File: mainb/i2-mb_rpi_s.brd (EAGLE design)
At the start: 110 x 106.6 mm, 27 parts, among them IC3 DS1307Z, T1 BC337, T2 BC337, X9 eth (mb->rpi)

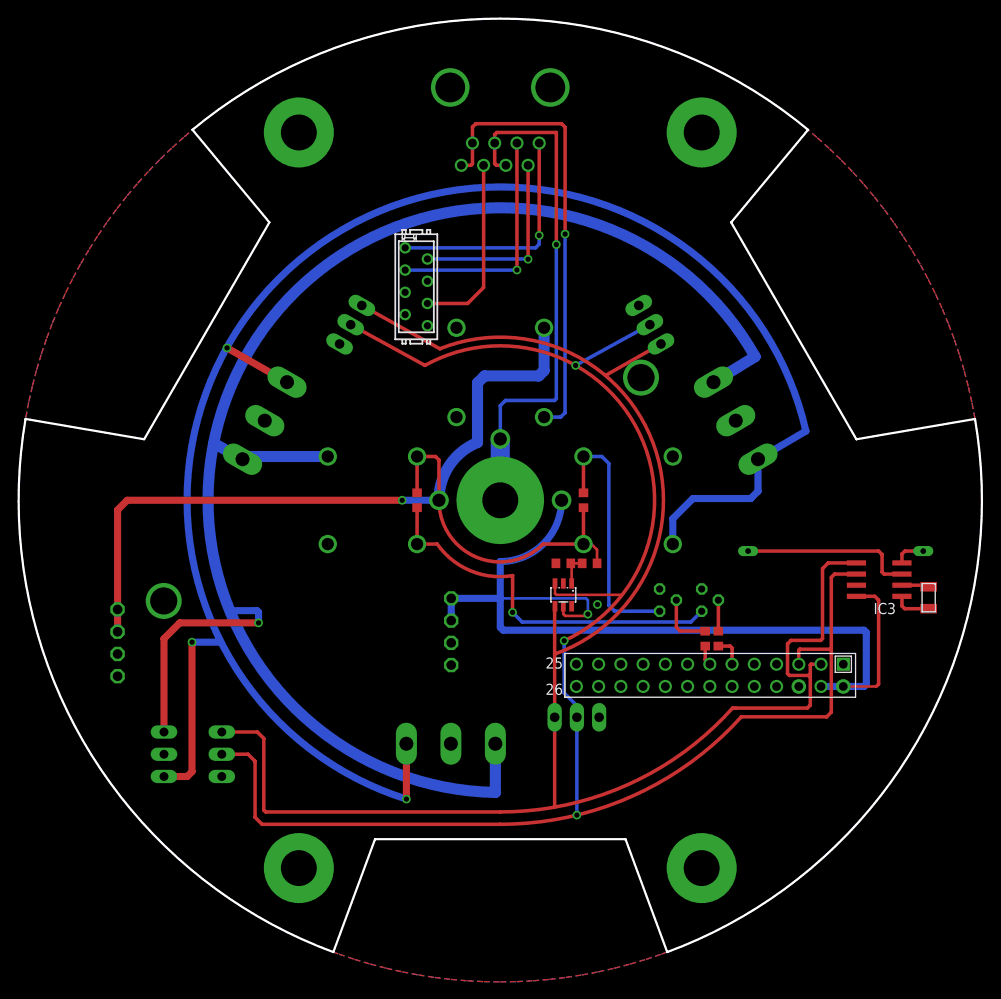
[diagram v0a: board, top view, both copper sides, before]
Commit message: 22.11.13 17:00
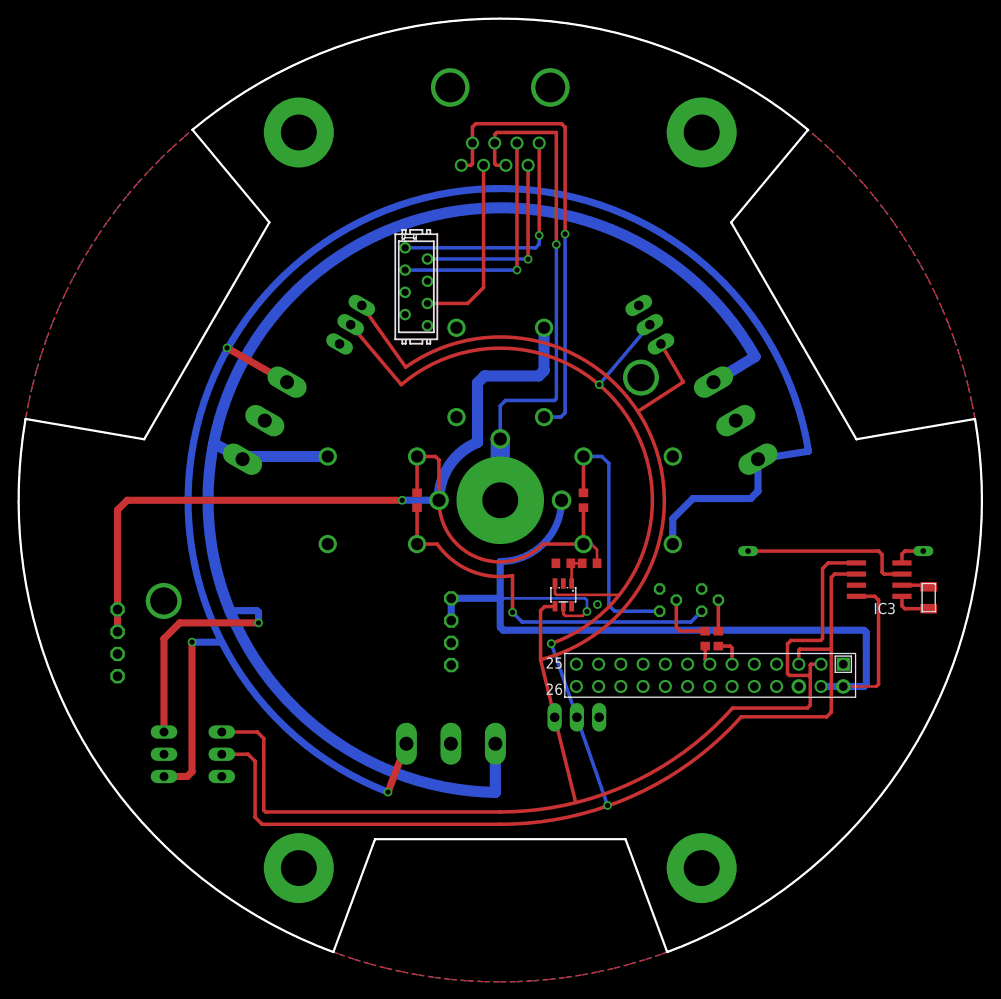
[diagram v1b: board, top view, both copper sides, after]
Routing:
- net SCL: track 200.5 -> 183.5 mm
- net SDA: track 184.4 -> 187.6 mm
- net +5V: track 121.6 -> 120.5 mm
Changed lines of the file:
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@@
 <layer number="46" name="Milling" color="3" fill="1" visible="no" active="yes"/>
 <layer number="47" name="Measures" color="7" fill="1" visible="no" active="yes"/>
-<layer number="48" name="Document" color="7" fill="1" visible="no" active="yes"/>
+<layer number="48" name="Document" color="7" fill="1" visible="yes" active="yes"/>
 <layer number="49" name="Reference" color="7" fill="1" visible="yes" active="yes"/>
 <layer number="50" name="dxf" color="7" fill="1" visible="no" active="no"/>
@@
 <contactref element="I2C_3" pad="2"/>
 <contactref element="I2C_4" pad="2"/>
-<wire x1="-17.0808875" y1="20.049996875" x2="-8.6" y2="15.4" width="0.4064" layer="1"/>
-<wire x1="8.75" y1="-24.78" x2="8.75" y2="-23.45" width="0.4064" layer="16"/>
-<wire x1="7.3" y1="-22" x2="7.3" y2="-16.04" width="0.4064" layer="16"/>
-<wire x1="-8.6" y1="15.4" x2="8.6" y2="15.4" width="0.4064" layer="1" curve="-58.361612"/>
-<wire x1="17.0808875" y1="20.05" x2="8.6" y2="15.4" width="0.4064" layer="16"/>
-<via x="8.6" y="15.4" extent="1-16" drill="0.6"/>
-<wire x1="8.6" y1="15.4" x2="7.3" y2="-16.04" width="0.4064" layer="1" curve="-126.269"/>
-<wire x1="7.3" y1="-22" x2="8.75" y2="-23.45" width="0.4064" layer="16"/>
-<via x="7.3" y="-16.04" extent="1-16" drill="0.6"/>
 <contactref element="I2C_1" pad="2"/>
 <wire x1="-31.8" y1="-29" x2="-28.8" y2="-29" width="0.4064" layer="1"/>
@@
 <wire x1="6.25" y1="-9.4999" x2="6.25" y2="-10.65" width="0.3048" layer="1"/>
 <wire x1="6.25" y1="-10.65" x2="6.4" y2="-10.8" width="0.3048" layer="1"/>
-<wire x1="6.4" y1="-10.8" x2="13.8" y2="-10.8" width="0.3048" layer="1"/>
+<wire x1="6.4" y1="-10.8" x2="13.6" y2="-10.8" width="0.3048" layer="1"/>
 <wire x1="34.09" y1="-18.72" x2="34.09" y2="-17.11" width="0.4064" layer="1"/>
 <wire x1="34.09" y1="-17.11" x2="34.2" y2="-17" width="0.4064" layer="1"/>
 <wire x1="34.2" y1="-17" x2="37.8" y2="-17" width="0.4064" layer="1"/>
 <wire x1="37.8" y1="-17" x2="37.8" y2="-24.2" width="0.4064" layer="1"/>
-<wire x1="8.75" y1="-24.78" x2="8.75" y2="-35.85" width="0.4064" layer="16"/>
+<wire x1="8.75" y1="-24.78" x2="12.25" y2="-34.85" width="0.4064" layer="16"/>
 <wire x1="37.27" y1="-24.73" x2="27.52" y2="-24.73" width="0.4064" layer="1"/>
 <wire x1="0" y1="-37" x2="27.52" y2="-24.73" width="0.4064" layer="1" curve="48.0587"/>
@@
 <wire x1="37.8" y1="-8.8" x2="38.175" y2="-8.425" width="0.4064" layer="1"/>
 <wire x1="40.67" y1="-8.425" x2="38.175" y2="-8.425" width="0.4064" layer="1"/>
-<via x="8.75" y="-35.95" extent="1-16" drill="0.6"/>
-<wire x1="8.75" y1="-35.85" x2="8.75" y2="-35.95" width="0" layer="19" extent="16-16"/>
-<wire x1="6.4" y1="-10.8" x2="7.3" y2="-16.04" width="0" layer="19" extent="1-16"/>
-<wire x1="0" y1="-37" x2="8.75" y2="-35.95" width="0" layer="19" extent="1-1"/>
+<via x="12.25" y="-34.85" extent="1-16" drill="0.6"/>
+<wire x1="-17.0808875" y1="20.049996875" x2="-11.3" y2="13.2" width="0.4064" layer="1"/>
+<wire x1="17.0808875" y1="20.05" x2="11.3" y2="13.2" width="0.4064" layer="16"/>
+<wire x1="8.75" y1="-24.78" x2="5.82" y2="-16.37" width="0.4064" layer="16"/>
+<wire x1="-11.3" y1="13.2" x2="5.82" y2="-16.37" width="0.4064" layer="1" curve="-200.979"/>
+<via x="5.82" y="-16.37" extent="1-16" drill="0.6"/>
+<via x="11.3" y="13.2" extent="1-16" drill="0.6"/>
+<wire x1="-11.3" y1="13.2" x2="11.3" y2="13.2" width="0" layer="19" extent="1-16"/>
+<wire x1="6.4" y1="-10.8" x2="5.82" y2="-16.37" width="0" layer="19" extent="1-16"/>
+<wire x1="0" y1="-37" x2="12.25" y2="-34.85" width="0" layer="19" extent="1-1"/>
 </signal>
 <signal name="SDA">
@@
 <contactref element="I2C_3" pad="1"/>
 <contactref element="I2C_4" pad="1"/>
-<wire x1="6.21" y1="-24.78" x2="6.21" y2="-17.5650875" width="0.4064" layer="1"/>
-<wire x1="6.21" y1="-17.5650875" x2="6.21" y2="-12.1401" width="0.4064" layer="1"/>
-<wire x1="-15.8108875" y1="22.249703125" x2="-6.9" y2="17.3" width="0.4064" layer="1"/>
-<wire x1="18.3508875" y1="17.85029375" x2="12.1" y2="14.3" width="0.4064" layer="1"/>
-<wire x1="-6.9" y1="17.3" x2="6.21" y2="-17.5650875" width="0.4064" layer="1" curve="-182.32"/>
 <contactref element="I2C_1" pad="1"/>
 <wire x1="-31.8" y1="-26.46" x2="-27.74" y2="-26.46" width="0.4064" layer="1"/>
@@
 <wire x1="35.4" y1="-18.8" x2="35.4" y2="-20.2" width="0.4064" layer="1"/>
 <wire x1="35.4" y1="-20.2" x2="35.4" y2="-23.4" width="0.4064" layer="1"/>
-<wire x1="35.07" y1="-23.73" x2="26.92" y2="-23.73" width="0.4064" layer="1"/>
+<wire x1="35.07" y1="-23.73" x2="26.524365625" y2="-23.73" width="0.4064" layer="1"/>
 <wire x1="0" y1="-35.59" x2="26.5231375" y2="-23.731228125" width="0.4064" layer="1" curve="48.17983"/>
 <wire x1="35.07" y1="-23.73" x2="35.4" y2="-23.4" width="0.4064" layer="1"/>
-<wire x1="6.21" y1="-24.78" x2="6.21" y2="-34.99" width="0.4064" layer="1"/>
-<wire x1="6.21" y1="-34.99" x2="6.2" y2="-35" width="0.4064" layer="1"/>
+<wire x1="6.21" y1="-24.78" x2="8.61" y2="-34.49" width="0.4064" layer="1"/>
 <wire x1="33" y1="-20" x2="35.2" y2="-20" width="0.4064" layer="1"/>
 <wire x1="35.2" y1="-20" x2="35.4" y2="-20.2" width="0.4064" layer="1"/>
@@
 <wire x1="36.8" y1="-7.8" x2="37.445" y2="-7.155" width="0.4064" layer="1"/>
 <wire x1="40.67" y1="-7.155" x2="37.445" y2="-7.155" width="0.4064" layer="1"/>
-<wire x1="26.92" y1="-23.73" x2="26.524365625" y2="-23.73" width="0.4064" layer="1"/>
 <wire x1="26.524365625" y1="-23.73" x2="26.5231375" y2="-23.731228125" width="0.3048" layer="1"/>
-<wire x1="-6.9" y1="17.3" x2="12.1" y2="14.3" width="0" layer="19" extent="1-1"/>
-<wire x1="0" y1="-35.59" x2="6.21" y2="-34.99" width="0" layer="19" extent="1-1"/>
+<wire x1="-15.8108875" y1="22.249703125" x2="-10.8" y2="15.2" width="0.4064" layer="1"/>
+<wire x1="6.21" y1="-24.78" x2="4.6" y2="-18.2" width="0.4064" layer="1"/>
+<wire x1="-10.8" y1="15.2" x2="4.6" y2="-18.2" width="0.4064" layer="1" curve="-201.211"/>
+<wire x1="6.21" y1="-12.1401" x2="5.0599" y2="-12.1401" width="0.4064" layer="1"/>
+<wire x1="5.0599" y1="-12.1401" x2="4.6" y2="-12.6" width="0.4064" layer="1"/>
+<wire x1="4.6" y1="-12.6" x2="4.6" y2="-18.2" width="0.4064" layer="1"/>
+<wire x1="18.3508875" y1="17.85029375" x2="20.9" y2="13.5" width="0.4064" layer="1"/>
+<wire x1="20.9" y1="13.5" x2="15.8" y2="10.2" width="0.4064" layer="1"/>
+<wire x1="6.25" y1="-12.1001" x2="15.8" y2="10.2" width="0" layer="19" extent="1-1"/>
+<wire x1="0" y1="-35.59" x2="8.61" y2="-34.49" width="0" layer="19" extent="1-1"/>
 </signal>
 <signal name="N$41">
@@
 <contactref element="T1" pad="3"/>
 <wire x1="-9.5" y1="-0.85" x2="-9.5" y2="-5" width="0.4064" layer="1"/>
-<wire x1="1.4" y1="-12.8" x2="1.41" y2="-8.6" width="0.4064" layer="1"/>
+<wire x1="1.4" y1="-12.8" x2="1.4" y2="-8.6" width="0.4064" layer="1"/>
 <via x="1.4" y="-12.8" extent="1-16" drill="0.6"/>
 <wire x1="-9.5" y1="-5" x2="-7.2" y2="-5" width="0.4064" layer="1"/>
-<wire x1="-7.2" y1="-5" x2="1.41" y2="-8.6" width="0.4064" layer="1" curve="64.4683"/>
+<wire x1="-7.2" y1="-5" x2="1.4" y2="-8.6" width="0.4064" layer="1" curve="64.4683"/>
 <wire x1="21.77" y1="-13.9" x2="2.5" y2="-13.9" width="0.4064" layer="16"/>
 <wire x1="2.5" y1="-13.9" x2="1.4" y2="-12.8" width="0.4064" layer="16"/>
@@
 <contactref element="PWR2" pad="1"/>
 <contactref element="PWR1" pad="1"/>
-<wire x1="-10.72" y1="-27.8" x2="-10.72" y2="-34.12" width="0.8128" layer="1"/>
-<wire x1="29.43" y1="4.690590625" x2="34.9" y2="7.9" width="0.8128" layer="16"/>
-<wire x1="-10.72" y1="-34.12" x2="34.9" y2="7.9" width="0.8128" layer="16" curve="-239.803468"/>
-<via x="-10.72" y="-34.12" extent="1-16" drill="0.6"/>
+<wire x1="-10.72" y1="-27.8" x2="-12.82" y2="-33.32" width="0.8128" layer="1"/>
+<wire x1="29.43" y1="4.690590625" x2="35.2" y2="5.6" width="0.8128" layer="16"/>
+<wire x1="-12.82" y1="-33.32" x2="35.2" y2="5.6" width="0.8128" layer="16" curve="-239.803468"/>
+<via x="-12.82" y="-33.32" extent="1-16" drill="0.6"/>
 <wire x1="-24.35" y1="13.48940625" x2="-31.2" y2="17.4" width="0.8128" layer="1"/>
 <via x="-31.2" y="17.4" extent="1-16" drill="0.6"/>
@@
 <via x="-35.2" y="-16.2" extent="1-16" drill="0.6"/>
 <wire x1="-35.2" y1="-16.2" x2="-32" y2="-16.2" width="0.8128" layer="16"/>
-<wire x1="-10.72" y1="-27.8" x2="-32" y2="-16.2" width="0" layer="19" extent="16-16"/>
+<wire x1="-12.82" y1="-33.32" x2="-35.2" y2="-31" width="0" layer="19" extent="1-1"/>
 <wire x1="-24.35" y1="13.48940625" x2="-32" y2="-16.2" width="0" layer="19" extent="16-16"/>
 </signal>
@@
 <wire x1="7.2" y1="-12.0999" x2="7.2" y2="-13" width="0.3048" layer="1"/>
 <wire x1="7.2" y1="-13" x2="7.4" y2="-13.2" width="0.3048" layer="1"/>
-<wire x1="7.4" y1="-13.2" x2="9.8" y2="-13.2" width="0.3048" layer="1"/>
-<wire x1="9.8" y1="-13.2" x2="10" y2="-13" width="0.3048" layer="1"/>
-<via x="10" y="-13" extent="1-16" drill="0.6"/>
-<wire x1="10" y1="-13" x2="10" y2="-11.4" width="0.3048" layer="16"/>
-<wire x1="10" y1="-11.4" x2="9.8" y2="-11.2" width="0.3048" layer="16"/>
-<wire x1="9.8" y1="-11.2" x2="0" y2="-11.2" width="0.3048" layer="16"/>
+<wire x1="7.4" y1="-13.2" x2="9.4" y2="-13.2" width="0.3048" layer="1"/>
+<wire x1="9.4" y1="-13.2" x2="9.9" y2="-12.7" width="0.3048" layer="1"/>
+<via x="9.9" y="-12.7" extent="1-16" drill="0.6"/>
+<wire x1="9.9" y1="-12.7" x2="9.9" y2="-11.4" width="0.3048" layer="16"/>
+<wire x1="9.9" y1="-11.4" x2="9.7" y2="-11.2" width="0.3048" layer="16"/>
+<wire x1="9.7" y1="-11.2" x2="0" y2="-11.2" width="0.3048" layer="16"/>
 <wire x1="40.67" y1="-10.965" x2="42.765" y2="-10.965" width="0.4064" layer="1"/>
 <wire x1="42.765" y1="-10.965" x2="43.2" y2="-11.4" width="0.4064" layer="1"/>
